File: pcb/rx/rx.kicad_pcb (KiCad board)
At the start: 2 copper layers, 53 parts, among them U1 nice_nano, U2 MPU-6500, U3 QMC5883P, U4 MCP6004, U5 MCP6004, U6 74HC4051

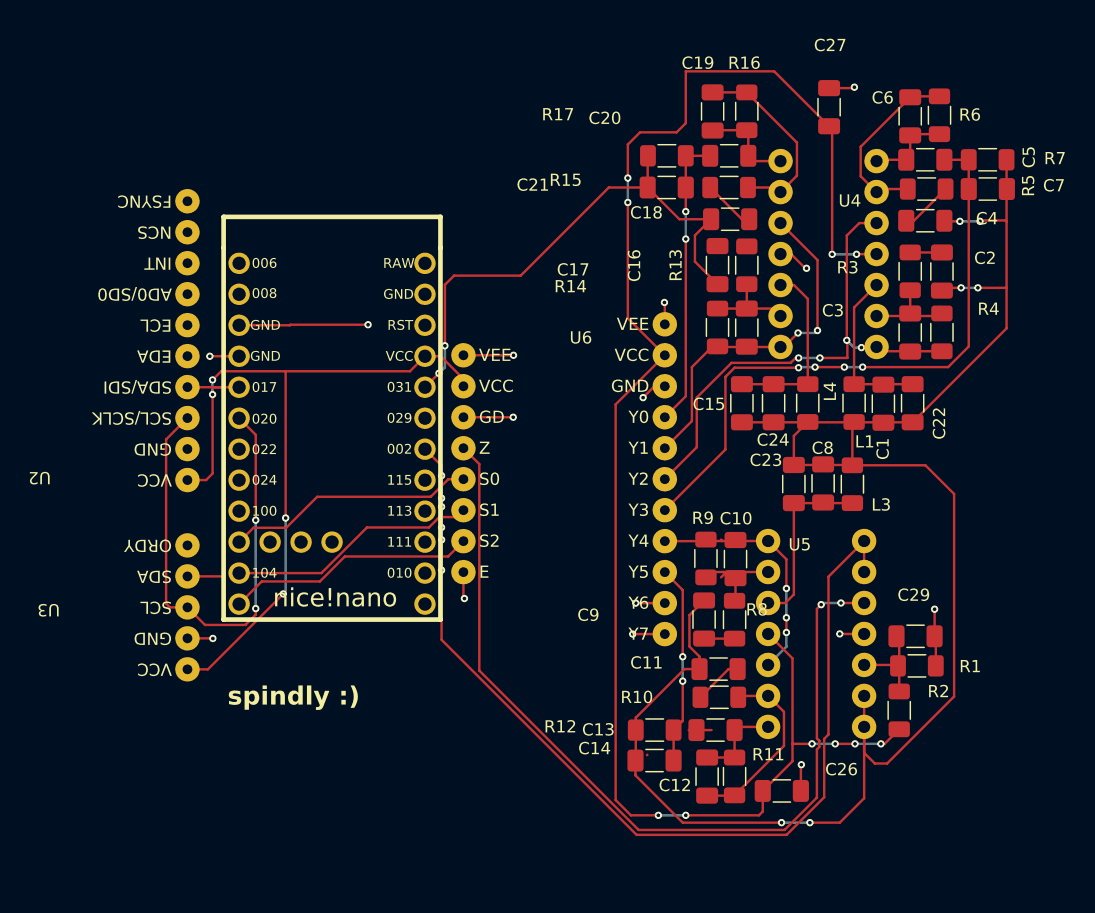
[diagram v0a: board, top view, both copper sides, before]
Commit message: Finished Rx
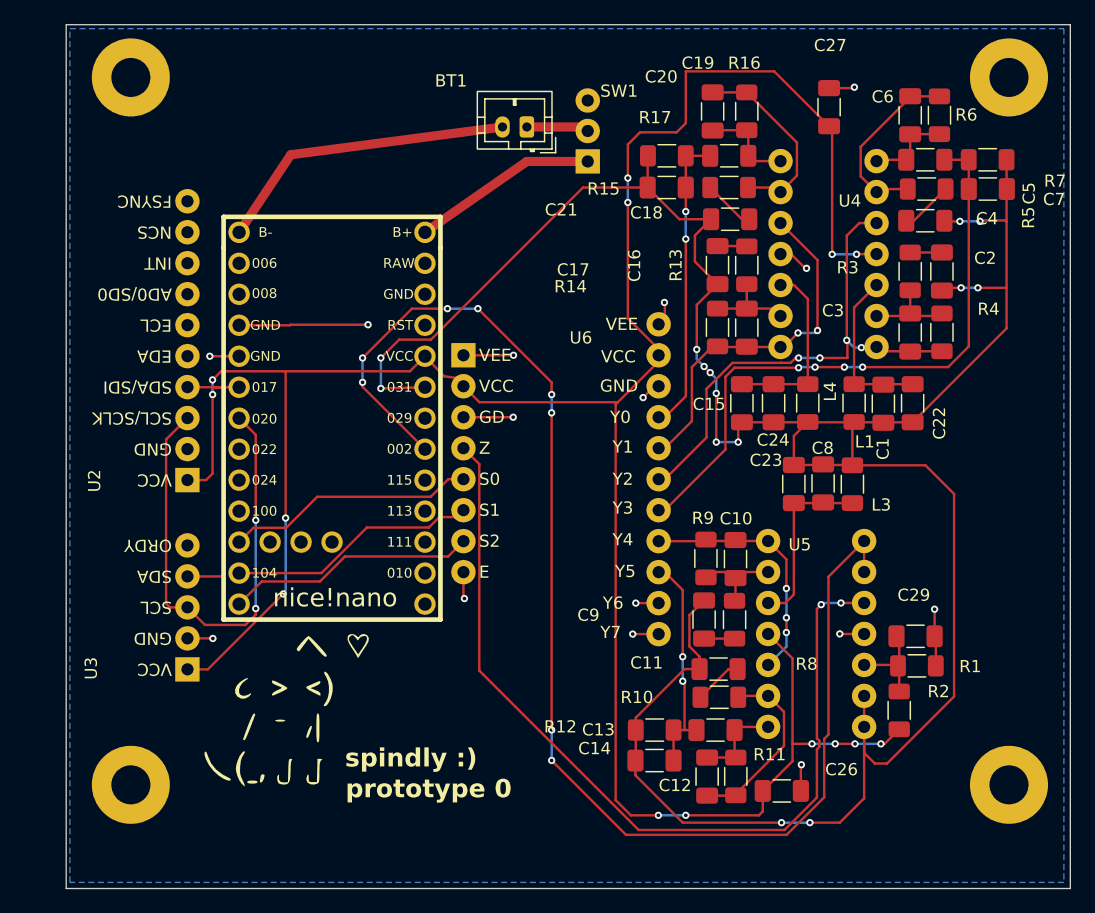
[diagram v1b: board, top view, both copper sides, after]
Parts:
- added BT1: Battery, Connector_JST:JST_PH_B2B-PH-K_1x02_P2.00mm_Vertical, F.Cu at (118.5, 35.6)
- added G***: LOGO, Library:cat_silkscreen, F.Cu at (98.3, 83.4)
- added REF**: MountingHole_3.2mm_M3_Pad, MountingHole:MountingHole_3.2mm_M3_Pad, F.Cu at (158.0, 31.5)
- added REF**: MountingHole_3.2mm_M3_Pad, MountingHole:MountingHole_3.2mm_M3_Pad, F.Cu at (86.0, 89.5)
- added REF**: MountingHole_3.2mm_M3_Pad, MountingHole:MountingHole_3.2mm_M3_Pad, F.Cu at (86.0, 31.5)
- added REF**: MountingHole_3.2mm_M3_Pad, MountingHole:MountingHole_3.2mm_M3_Pad, F.Cu at (158.0, 89.5)
- added SW1: SW_SPDT, Library:EG1218, F.Cu at (121.5, 41.7)
- moved R11 0.10 mm to (135.6, 88.8)
- moved C6 0.09 mm to (149.9, 34.6)
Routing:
- net /ADC_0: track 80.4 -> 111.4 mm, vias 6 -> 8
- net /B-: track 0.00 -> 25.1 mm
- net /V_BIAS: track 191.9 -> 214.7 mm, vias 8 -> 14
- net /B+: track 0.00 -> 15.2 mm
- net +3.3V: track 194.1 -> 207.2 mm
- net Net-(BT1-+): track 0.00 -> 5.13 mm
- net Net-(C16-Pad1): track 0.00 -> 2.41 mm
- net Net-(U5A--): track 7.17 -> 6.55 mm
- added copper zone on B.Cu, net GND
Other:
- board outline added: 82.3 x 70.8 mm
- board text added: "prototype 0"
